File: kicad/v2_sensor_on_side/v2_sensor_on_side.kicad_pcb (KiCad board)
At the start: 2 copper layers, 47.6 x 44.9 mm, 13 parts, among them SW1 SW_Push, SW2 SW_Push, U1 nice_nano, U2 GY-BNO08X, U3 SSD1306_OLED_042, U4 SSD1306_OLED_042

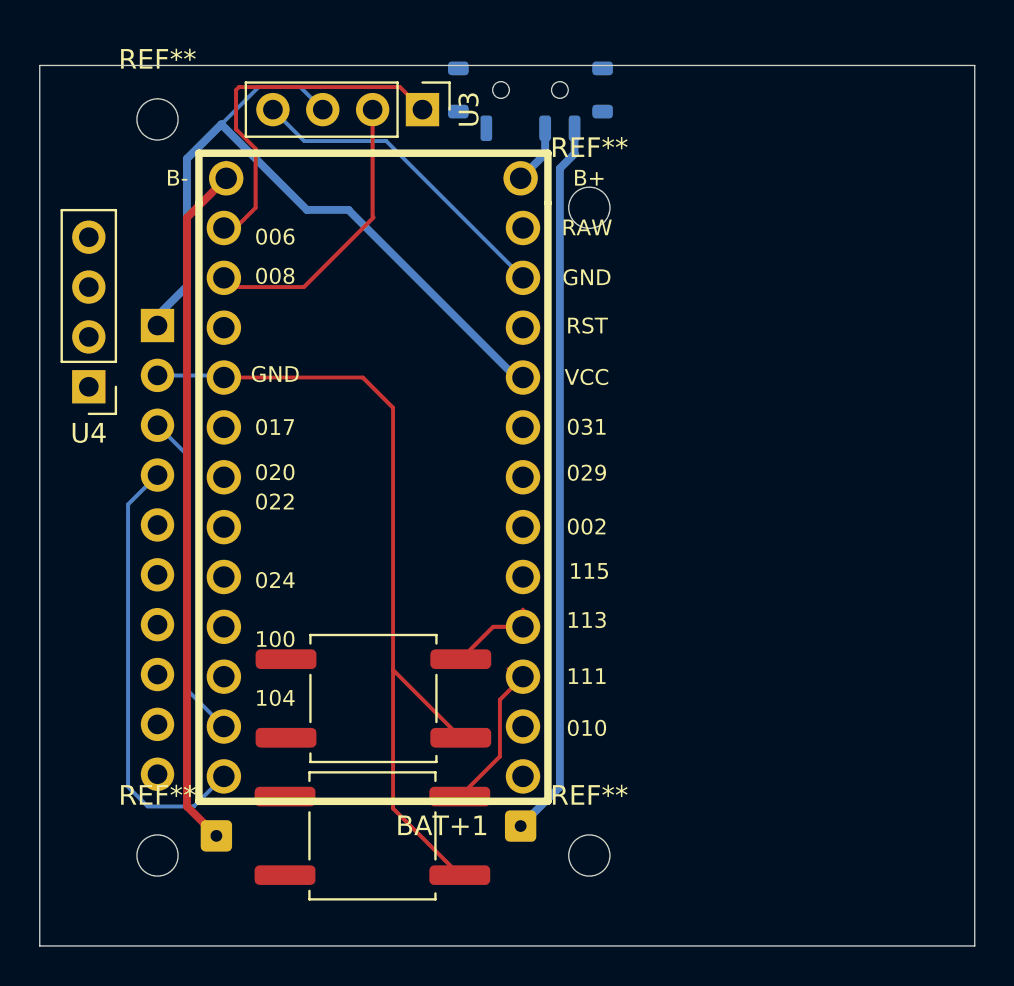
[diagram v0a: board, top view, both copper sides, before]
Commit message: kicad: tidy up
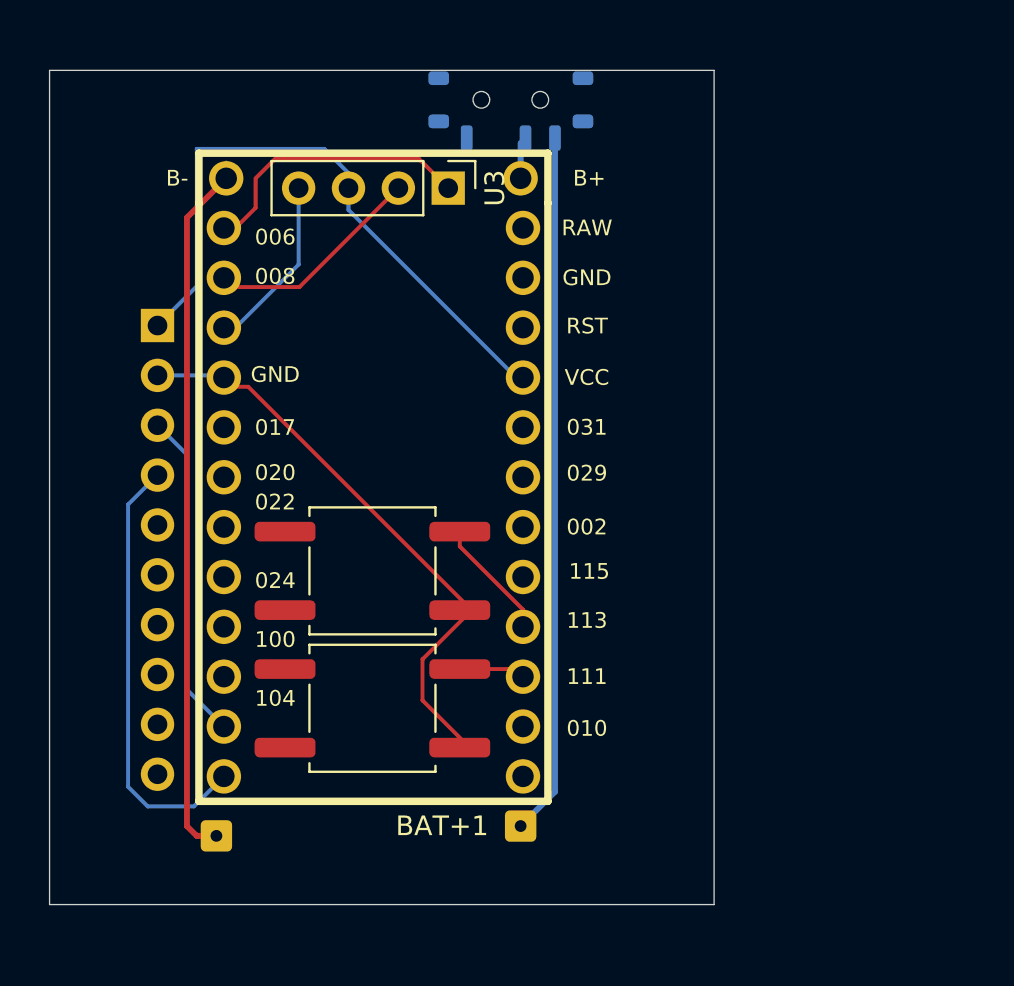
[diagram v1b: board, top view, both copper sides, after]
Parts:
- removed REF** (x4): MountingHole_2.1mm, MountingHole:MountingHole_2.1mm
- removed U4: SSD1306_OLED_042, Connector_PinHeader_2.54mm:PinHeader_1x04_P2.54mm_Vertical
- moved SW2 6.50 mm to (186.9, 72.0)
- moved SW1 6.50 mm to (186.9, 79.0)
- moved U3 4.21 mm to (190.8, 52.5)
- moved SW_POWER1 1.12 mm to (194.0, 48.0)
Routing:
- net GND: track 59.5 -> 39.2 mm
- net Net-(U1-VCC): track 39.1 -> 32.7 mm
- net Net-(U1-P1.11): track 9.21 -> 4.60 mm
- net Net-(U1-TX0/P0.06): track 18.6 -> 14.5 mm
- net Net-(U1-RX1/P0.08): track 14.5 -> 10.9 mm
- net Net-(U1-P1.13): track 4.73 -> 6.18 mm
- net Net-(BAT+1-Pin_1): track 36.2 -> 35.3 mm
- net Net-(BAT-1-Pin_1): track 36.9 -> 37.5 mm
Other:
- board size 47.6 x 44.9 mm -> 33.9 x 42.5 mm
